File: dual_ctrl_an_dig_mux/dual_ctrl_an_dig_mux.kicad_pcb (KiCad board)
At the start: 2 copper layers, 121 x 147 mm, 53 parts, among them J1 Conn_Coaxial, J10 Conn_Coaxial, J11 Conn_Coaxial, J12 Conn_Coaxial, J13 Conn_Coaxial, J14 Conn_Coaxial, J15 Conn_Coaxial, J16 Conn_Coaxial, J17 Conn_Coaxial, J18 Conn_Coaxial, J19 Conn_Coaxial, J20 Conn_Coaxial, J21 Conn_Coaxial, J22 Conn_Coaxial, J23 Conn_Coaxial, J24 Conn_Coaxial, J25 Conn_Coaxial, J26 Conn_Coaxial, J27 Conn_Coaxial, J28 Conn_Coaxial, J29 Conn_Coaxial, J3 Conn_Coaxial, J30 Conn_Coaxial, J31 Conn_Coaxial, J32 Conn_Coaxial, J33 Conn_Coaxial, J34 Conn_Coaxial, J35 Conn_Coaxial, J36 Conn_Coaxial, J37 Conn_Coaxial, J38 Conn_Coaxial, J39 Conn_Coaxial, J4 Conn_Coaxial, J40 Conn_Coaxial, J41 Conn_Coaxial, J42 Conn_Coaxial, J43 Conn_Coaxial, J44 Conn_Coaxial, J45 Conn_Coaxial, J5 Conn_Coaxial, J6 Conn_Coaxial, J7 Conn_Coaxial, J8 Conn_Coaxial, J9 Conn_Coaxial, U1 74HC157, U2 74HC157, U3 74HC4053, U4 74HC4053

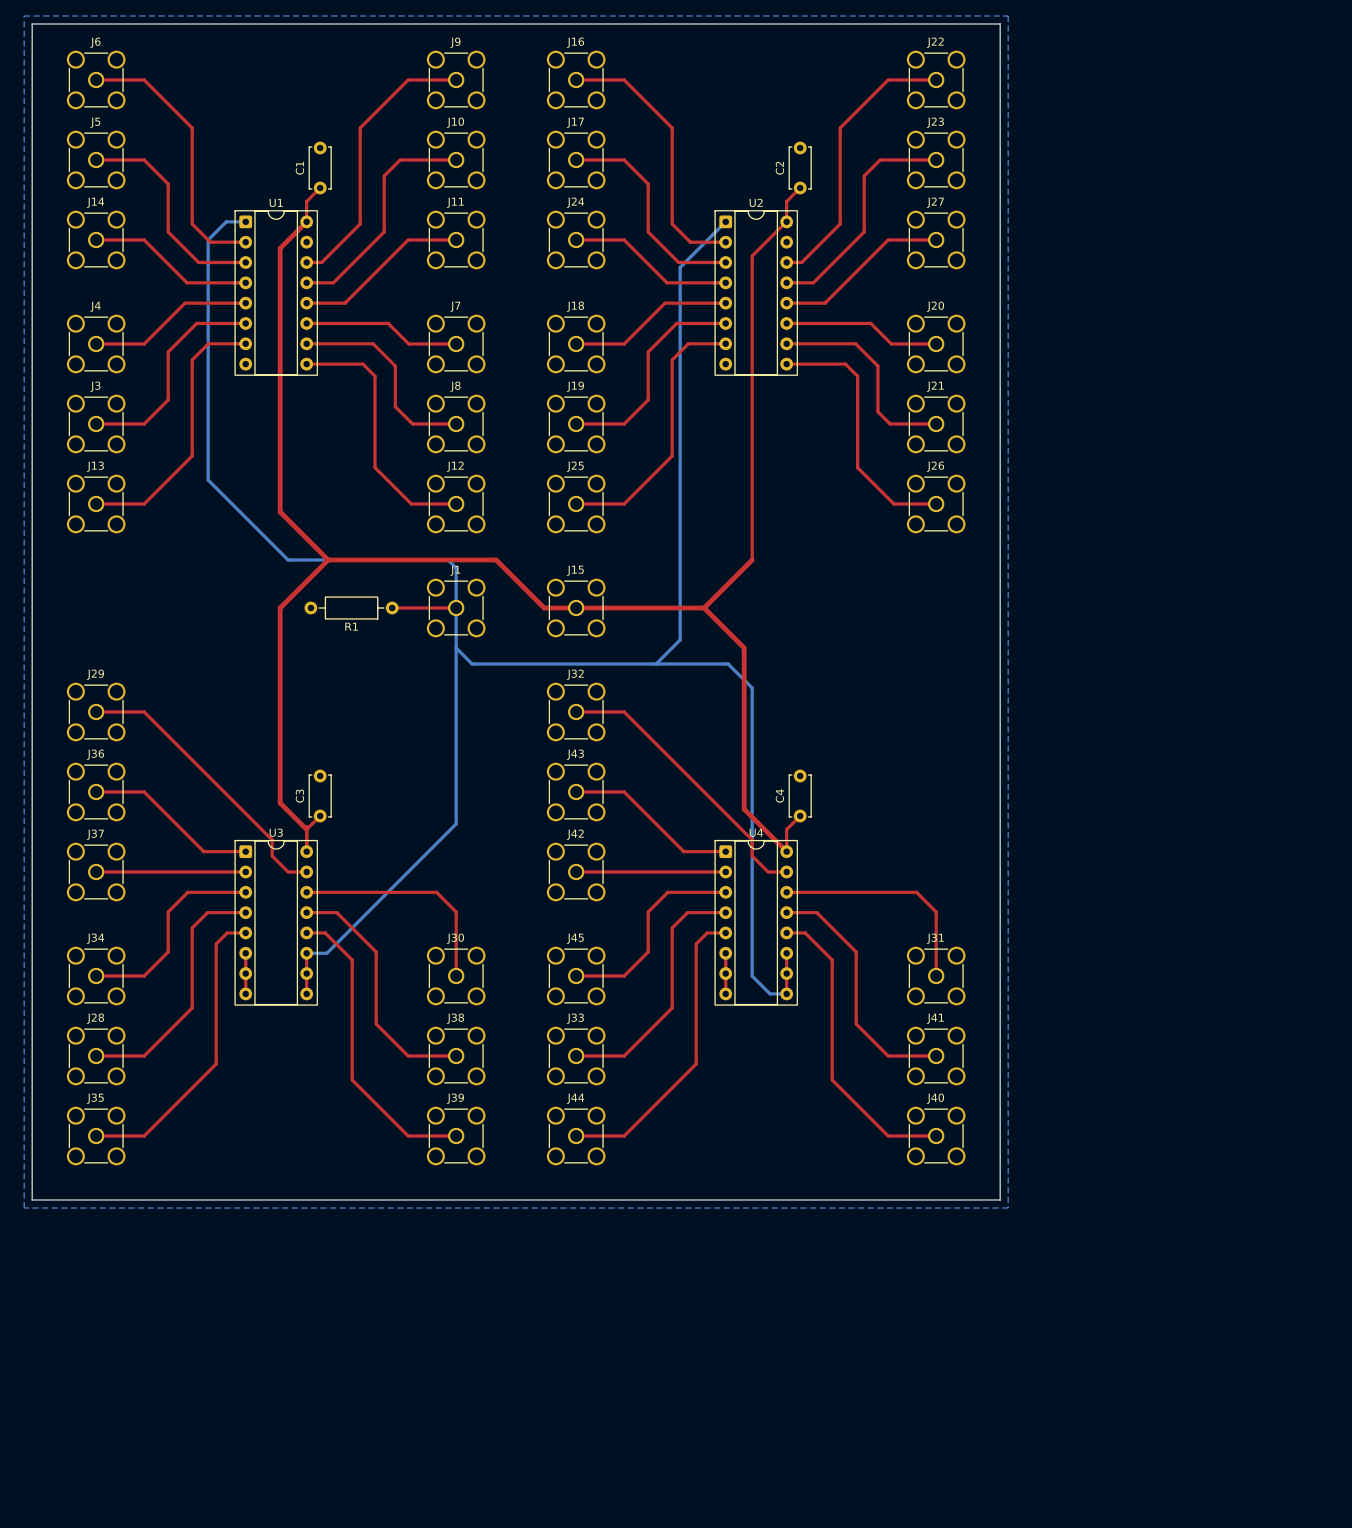
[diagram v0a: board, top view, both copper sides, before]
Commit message: Incorporated feedback from ABF
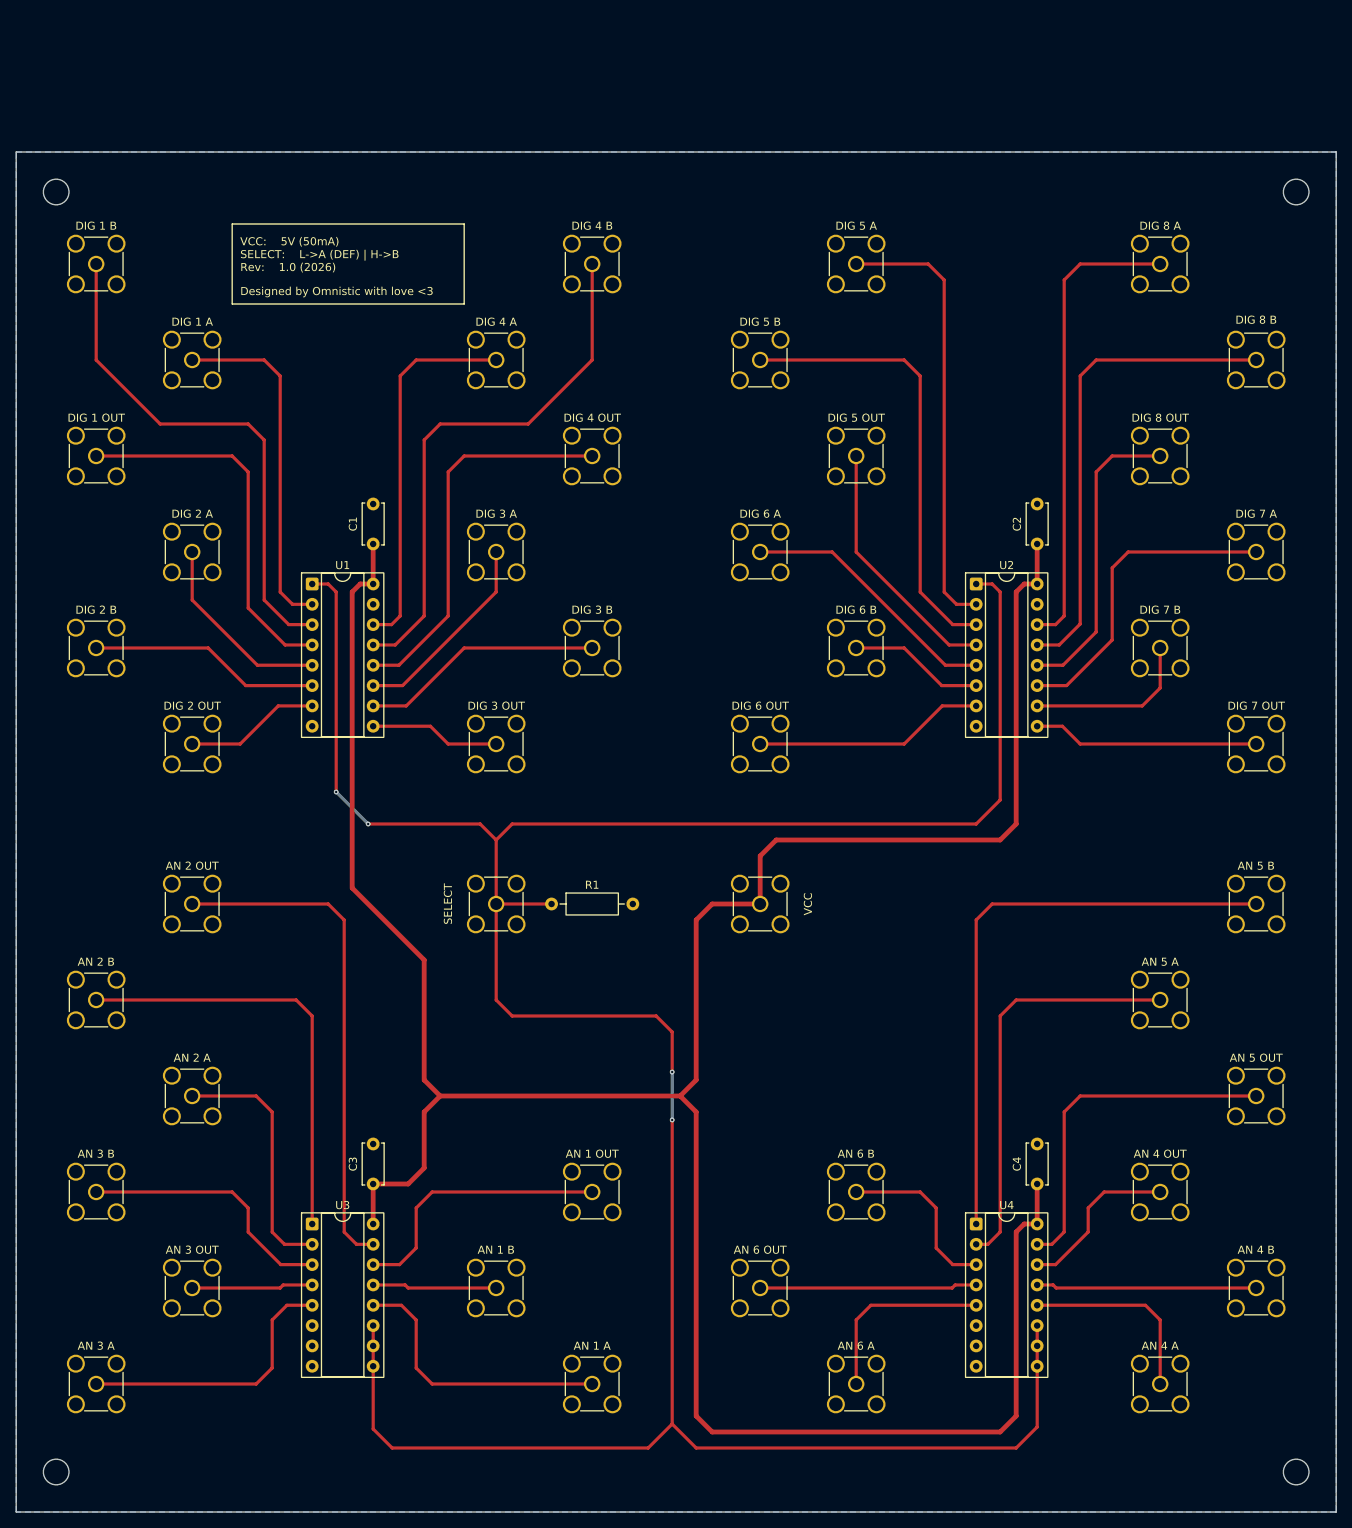
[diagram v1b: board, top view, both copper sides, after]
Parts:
- added REF**: MountingHole_3.2mm_M3, MountingHole:MountingHole_3.2mm_M3, F.Cu at (30.0, 40.0)
- added REF**: MountingHole_3.2mm_M3, MountingHole:MountingHole_3.2mm_M3, F.Cu at (185.0, 40.0)
- added REF**: MountingHole_3.2mm_M3, MountingHole:MountingHole_3.2mm_M3, F.Cu at (185.0, 200.0)
- added REF**: MountingHole_3.2mm_M3, MountingHole:MountingHole_3.2mm_M3, F.Cu at (30.0, 200.0)
- AN 1 A: renamed from J39
- AN 1 B: renamed from J38
- AN 1 OUT: renamed from J30
- AN 2 A: renamed from J37
- AN 2 B: renamed from J36
- AN 2 OUT: renamed from J29
- AN 3 A: renamed from J35
- AN 3 B: renamed from J34
- AN 3 OUT: renamed from J28
- AN 4 A: renamed from J40
- AN 4 B: renamed from J41
- AN 4 OUT: renamed from J31
- AN 5 A: renamed from J42
- AN 5 B: renamed from J43
- AN 5 OUT: renamed from J32
- AN 6 A: renamed from J44
- AN 6 B: renamed from J45
- AN 6 OUT: renamed from J33
- DIG 1 A: renamed from J6
- DIG 1 B: renamed from J5
- DIG 1 OUT: renamed from J14
- DIG 2 A: renamed from J4
- DIG 2 B: renamed from J3
- DIG 2 OUT: renamed from J13
- DIG 3 A: renamed from J7
- DIG 3 B: renamed from J8
- DIG 3 OUT: renamed from J12
- DIG 4 A: renamed from J9
- DIG 4 B: renamed from J10
- DIG 4 OUT: renamed from J11
- DIG 5 A: renamed from J16
- DIG 5 B: renamed from J17
- DIG 5 OUT: renamed from J24
- DIG 6 A: renamed from J18
- DIG 6 B: renamed from J19
- DIG 6 OUT: renamed from J25
- DIG 7 A: renamed from J20
- DIG 7 B: renamed from J21
- DIG 7 OUT: renamed from J26
- DIG 8 A: renamed from J22
- DIG 8 B: renamed from J23
- DIG 8 OUT: renamed from J27
- moved AN 5 OUT 97.6 mm to (180.0, 153.0)
- moved AN 5 B 86.1 mm to (180.0, 129.0)
- moved AN 5 A 74.7 mm to (168.0, 141.0)
- moved U4 56.1 mm to (145.0, 169.0)
- moved U2 55.0 mm to (145.0, 89.0)
- moved C4 54.7 mm to (152.6, 164.0)
- moved C2 53.5 mm to (152.6, 84.0)
- moved DIG 7 OUT 50.0 mm to (180.0, 109.0)
- moved AN 4 B 49.4 mm to (180.0, 177.0)
- moved DIG 7 A 47.7 mm to (180.0, 85.0)
- moved U3 47.3 mm to (62.0, 169.0)
- moved DIG 8 B 47.2 mm to (180.0, 61.0)
- moved AN 6 A 46.8 mm to (130.0, 189.0)
- moved C3 46.5 mm to (69.6, 164.0)
- moved U1 46.0 mm to (62.0, 89.0)
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- renumbered J1 to SELECT, J15 to VCC
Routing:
- net VCC: track 243.8 -> 350.0 mm
- net Net-(J1-In): track 285.9 -> 358.1 mm, vias 0 -> 4
- net Net-(J43-In): track 21.8 -> 73.8 mm
- net Net-(J10-In): track 29.2 -> 67.0 mm
- net Net-(J5-In): track 27.5 -> 64.4 mm
- net Net-(J42-In): track 18.7 -> 51.5 mm
- net Net-(J36-In): track 21.8 -> 53.8 mm
- net Net-(J23-In): track 29.2 -> 60.3 mm
- net Net-(J17-In): track 27.5 -> 56.5 mm
- net Net-(J29-In): track 35.8 -> 63.1 mm
- net Net-(J11-In): track 22.0 -> 48.8 mm
- net Net-(J14-In): track 20.9 -> 46.7 mm
- net Net-(J22-In): track 35.2 -> 58.7 mm
- net Net-(J16-In): track 34.1 -> 55.5 mm
- net Net-(J20-In): track 19.8 -> 39.6 mm
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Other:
- board size 121 x 147 mm -> 165 x 170 mm
- board text added: "Designed by Omnistic with love <3"
- board text added: "VCC: 5V (50mA) SELECT: L->A (DEF) | H->B Rev: 1.0 (2026)"
